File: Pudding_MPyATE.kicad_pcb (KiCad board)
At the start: 2 copper layers, 57 x 53.8 mm, 48 parts, among them J1 Conn_01x05_Pin, SW1 SW_Push, SW2 SW_Push, U1 LPC804M101JHI33, U2 TLV70233_SOT23-5, U3 LMV358

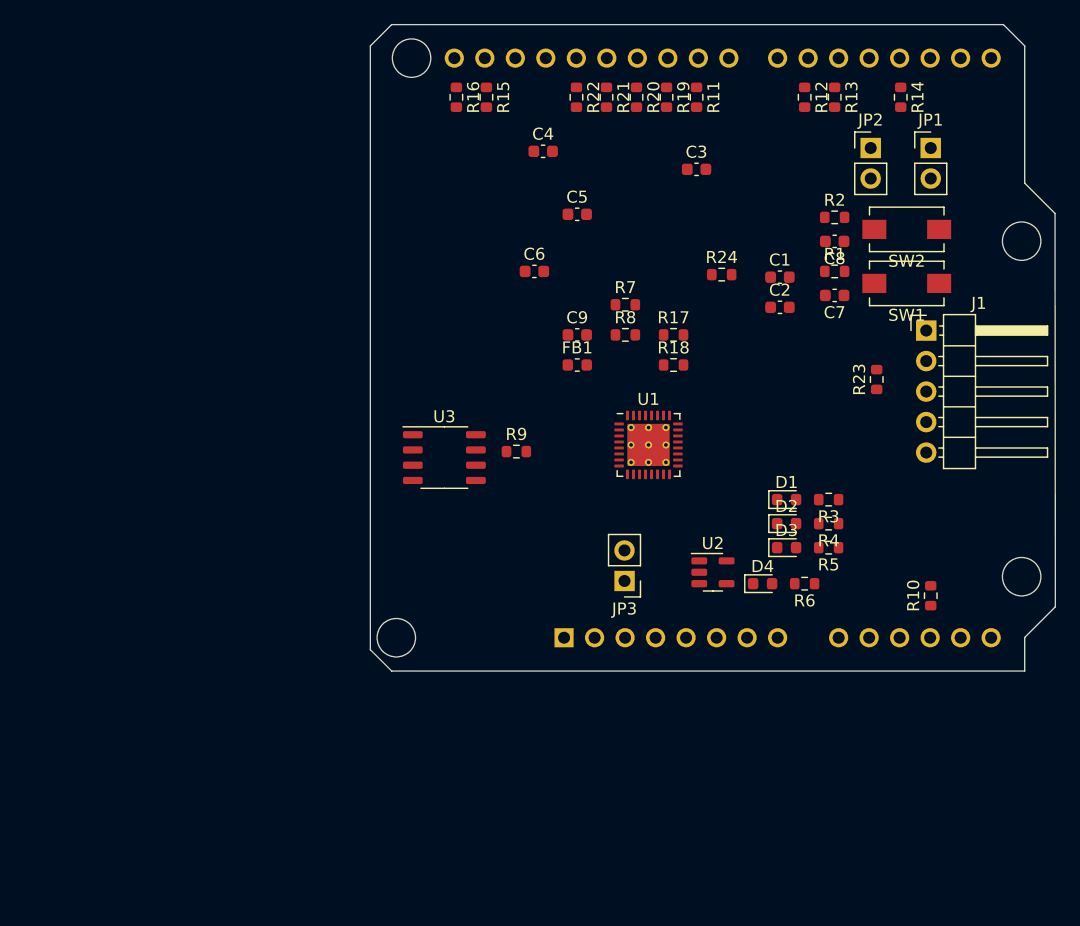
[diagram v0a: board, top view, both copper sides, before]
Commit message: Initial Rev. A0 signoff
Signed-off-by: Yilin Sun <imi415@imi.moe>
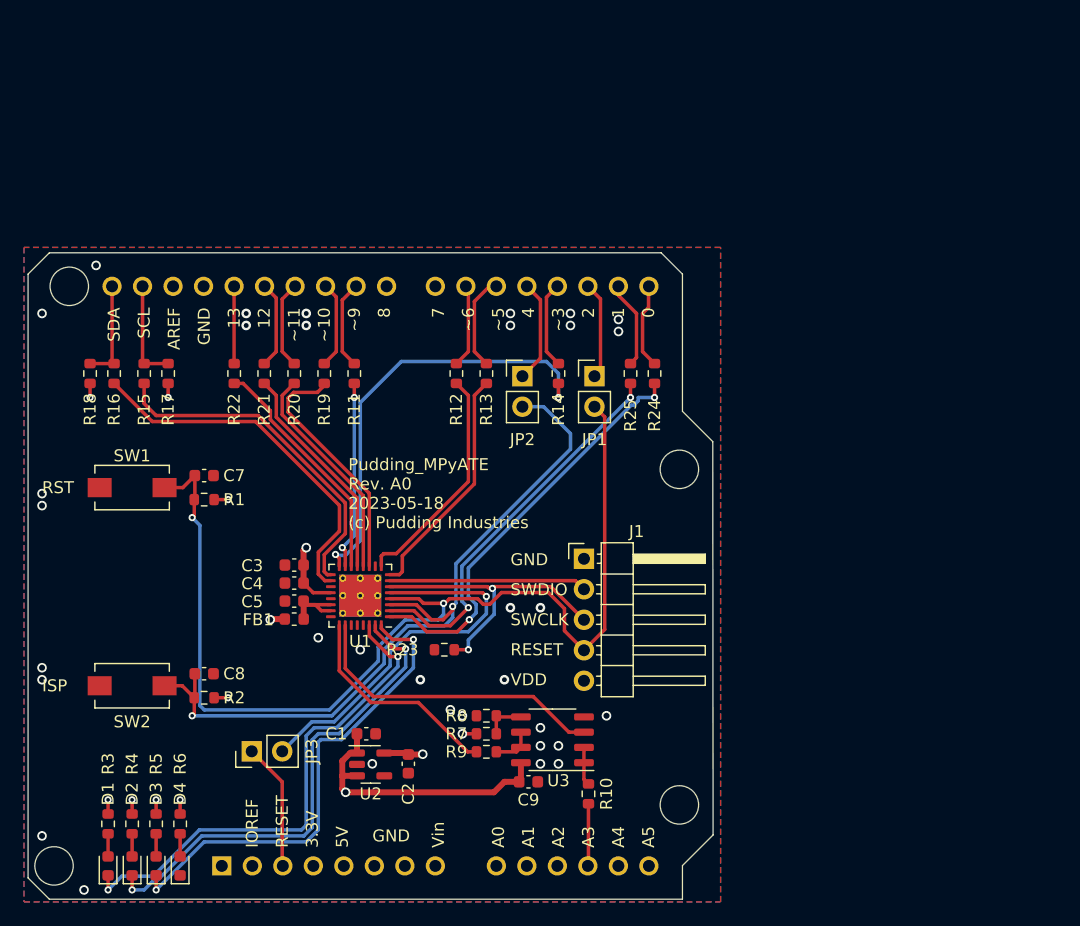
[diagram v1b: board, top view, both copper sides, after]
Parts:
- removed C6: 100nF, Capacitor_SMD:C_0603_1608Metric
- added R25: 100R, Resistor_SMD:R_0603_1608Metric, F.Cu at (168.0, 80.5)
- moved SW2 74.9 mm to (126.5, 106.5), turned to 0 degrees
- moved SW1 66.7 mm to (126.5, 90.0), turned to 0 degrees
- moved R2 66.0 mm to (132.5, 107.5), turned to 180 degrees
- moved R3 65.8 mm to (124.5, 118.0), turned to -90 degrees
- moved D1 64.2 mm to (124.5, 121.5), turned to 90 degrees
- moved C8 63.7 mm to (132.5, 105.5), turned to 0 degrees
- moved R4 63.2 mm to (126.5, 118.0), turned to -90 degrees
- moved D2 61.5 mm to (126.5, 121.5), turned to 90 degrees
- moved R5 60.5 mm to (128.5, 118.0), turned to -90 degrees
- moved D3 58.8 mm to (128.5, 121.5), turned to 90 degrees
- moved R1 55.8 mm to (132.5, 91.0), turned to 180 degrees
- moved R6 55.7 mm to (130.5, 118.0), turned to -90 degrees
- moved C7 54.6 mm to (132.5, 89.0), turned to 0 degrees
- moved D4 53.9 mm to (130.5, 121.5), turned to 90 degrees
- moved C1 51.3 mm to (146.0, 110.5)
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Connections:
- R24 pad 1: ARD_RST -> ARD_UART_RXD
- R24 pad 2: LPC_ARD_RST -> LPC_UART_RXD
- U1 pad 1: unconnected-(U1-PIO0_17/ADC_9-Pad1) -> LPC_UART_RXD
- U1 pad 11: LPC_SPI_SCK -> LPC_SPI_CS
- U1 pad 12: LPC_SPI_MISO -> LPC_SPI_MOSI
- U1 pad 13: LPC_SPI_MOSI -> LPC_SPI_MISO
- U1 pad 14: LPC_SPI_CS -> LPC_SPI_SCK
- U1 pad 15: LPC_LED_B -> LPC_IO3
- U1 pad 17: LPC_ADC_IOREF -> LPC_I2C_SCL
- U1 pad 18: LPC_IO2 -> LPC_I2C_SDA
- U1 pad 19: LPC_IO1 -> unconnected-(U1-PIO0_8/ADC_5-Pad19)
- U1 pad 2: unconnected-(U1-PIO0_13/ADC_10-Pad2) -> LPC_UART_TXD
- U1 pad 25: LPC_IO3 -> LPC_ADC_IOREF
- U1 pad 29: LPC_LED_R -> unconnected-(U1-PIO0_23-Pad29)
- U1 pad 30: LPC_LED_G -> LPC_LED_R
- U1 pad 31: unconnected-(U1-PIO0_18-Pad31) -> LPC_LED_G
- U1 pad 32: unconnected-(U1-PIO0_16/ADC_3/ACMP_I4-Pad32) -> LPC_LED_B
- U1 pad 8: LPC_I2C_SDA -> LPC_IO1
- U1 pad 9: LPC_I2C_SCL -> LPC_IO2
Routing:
- net LPC_RST: track 0.00 -> 89.3 mm, vias 0 -> 2
- net ARD_IOREF: track 0.00 -> 79.6 mm, vias 0 -> 3
- net LPC_ISP: track 0.00 -> 63.0 mm, vias 0 -> 2
- net LPC_LED_R: track 0.00 -> 42.2 mm, vias 0 -> 2
- net LPC_LED_G: track 0.00 -> 41.1 mm, vias 0 -> 2
- net LPC_LED_B: track 0.00 -> 40.3 mm, vias 0 -> 2
- net LPC_IO0: track 0.00 -> 36.7 mm, vias 0 -> 2
- net LPC_UART_RXD: track 0.00 -> 35.1 mm, vias 0 -> 2
- net LPC_UART_TXD: track 0.00 -> 32.4 mm, vias 0 -> 2
- net LPC_ARD_RST: track 0.00 -> 32.1 mm, vias 0 -> 1
- net LPC_I2C_SDA: track 0.00 -> 30.7 mm
- net +5V: track 0.00 -> 29.6 mm, vias 0 -> 1
- net LPC_I2C_SCL: track 0.00 -> 29.0 mm
- net LPC_DAC_OUT: track 0.00 -> 25.7 mm
- net LPC_SWCLK: track 0.00 -> 24.7 mm, vias 0 -> 2
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- added copper zone on B.Cu, net GND
- added copper zone on F.Cu, net GND
- added copper zone on In1.Cu, net GND
- added copper zone on In2.Cu, net VDD
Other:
- copper layers 2 -> 4
- board text added: "${TITLE} Rev. ${REVISION} ${ISSUE_DATE} (c) ${COMPANY}"
- board text added: "0"
- board text added: "1"
- board text added: "12"
- board text added: "13"
- board text added: "2"
- board text added: "3.3V"
- board text added: "4"
- board text added: "5V"
- board text added: "7"
- board text added: "8"
- board text added: "A0"
- board text added: "A1"
- board text added: "A2"
- board text added: "A3"
- board text added: "A4"
- board text added: "A5"
- board text added: "AREF"
- board text added: "GND"
- board text added: "IOREF"
- board text added: "ISP"
- board text added: "RESET"
- board text added: "RST"
- board text added: "SCL"
- board text added: "SDA"
- board text added: "SWCLK"
- board text added: "SWDIO"
- board text added: "VDD"
- board text added: "Vin"
- board text added: "~10"
- board text added: "~11"
- board text added: "~3"
- board text added: "~5"
- board text added: "~6"
- board text added: "~9"
